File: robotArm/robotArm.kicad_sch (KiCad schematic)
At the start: 17 parts, among them J1 Barrel_Jack, J2 ENDSTOP INPUTS, J3 STEPPER1, J4 STEPPER4, J5 STEPPER2, J6 STEPPER3, SW1 SW_DIP_x08, SW2 SW_SPDT, U2 TMC2209_SILENTSTEPSTICK, U4 TMC2209_MODULE, U5 TMC2209 Module

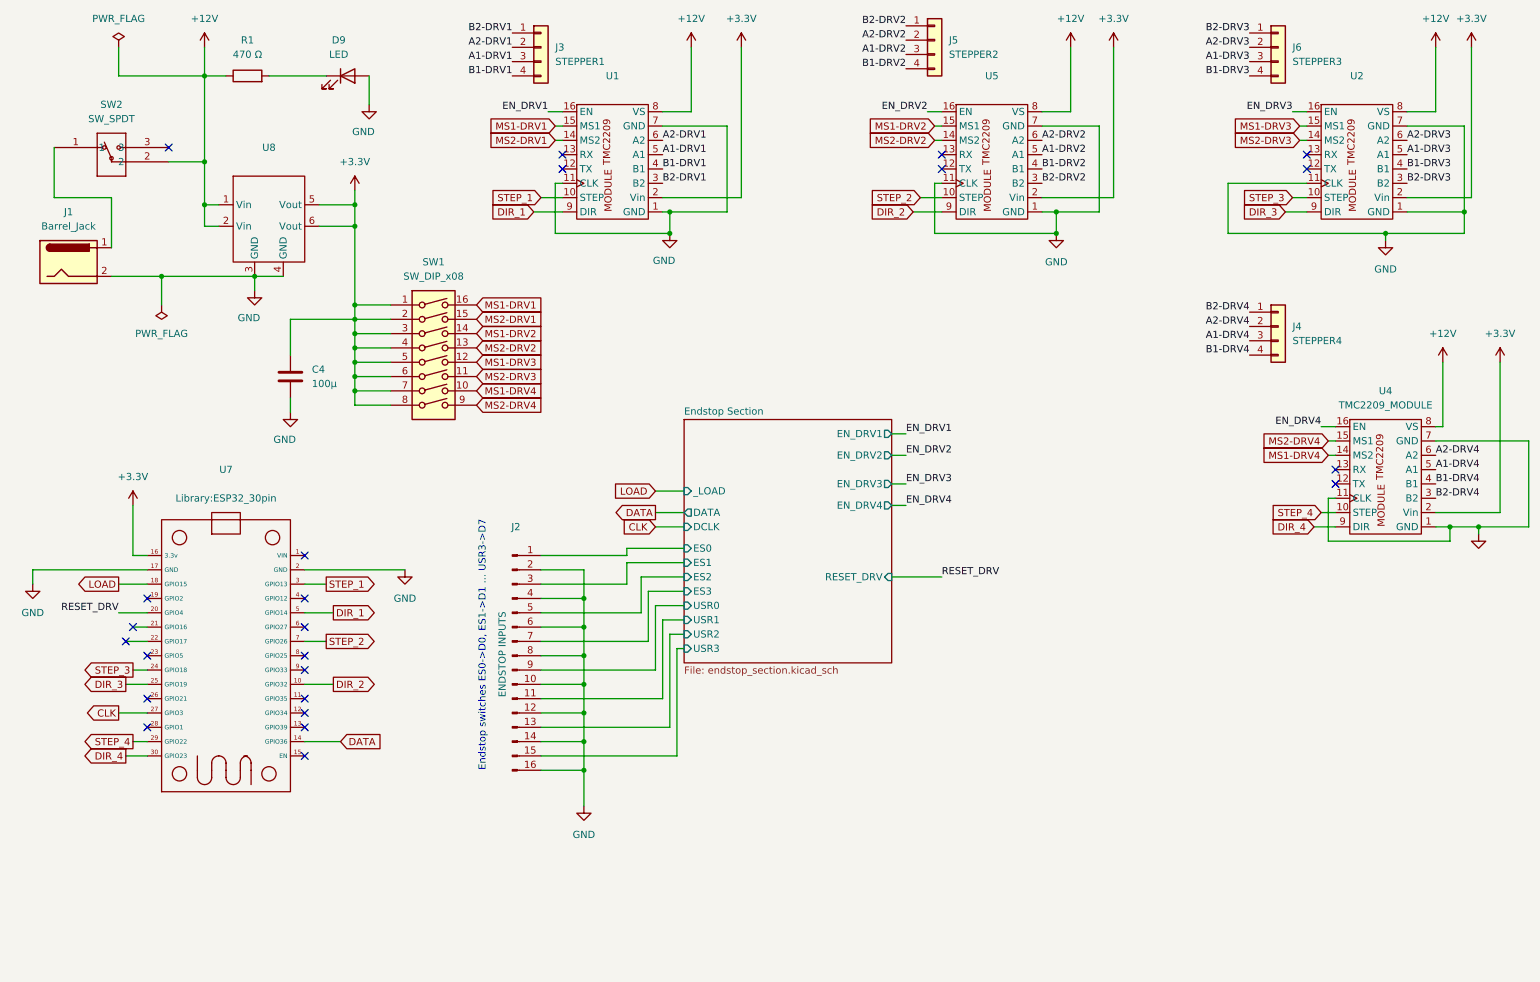
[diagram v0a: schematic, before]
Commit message: JLCPCB READY
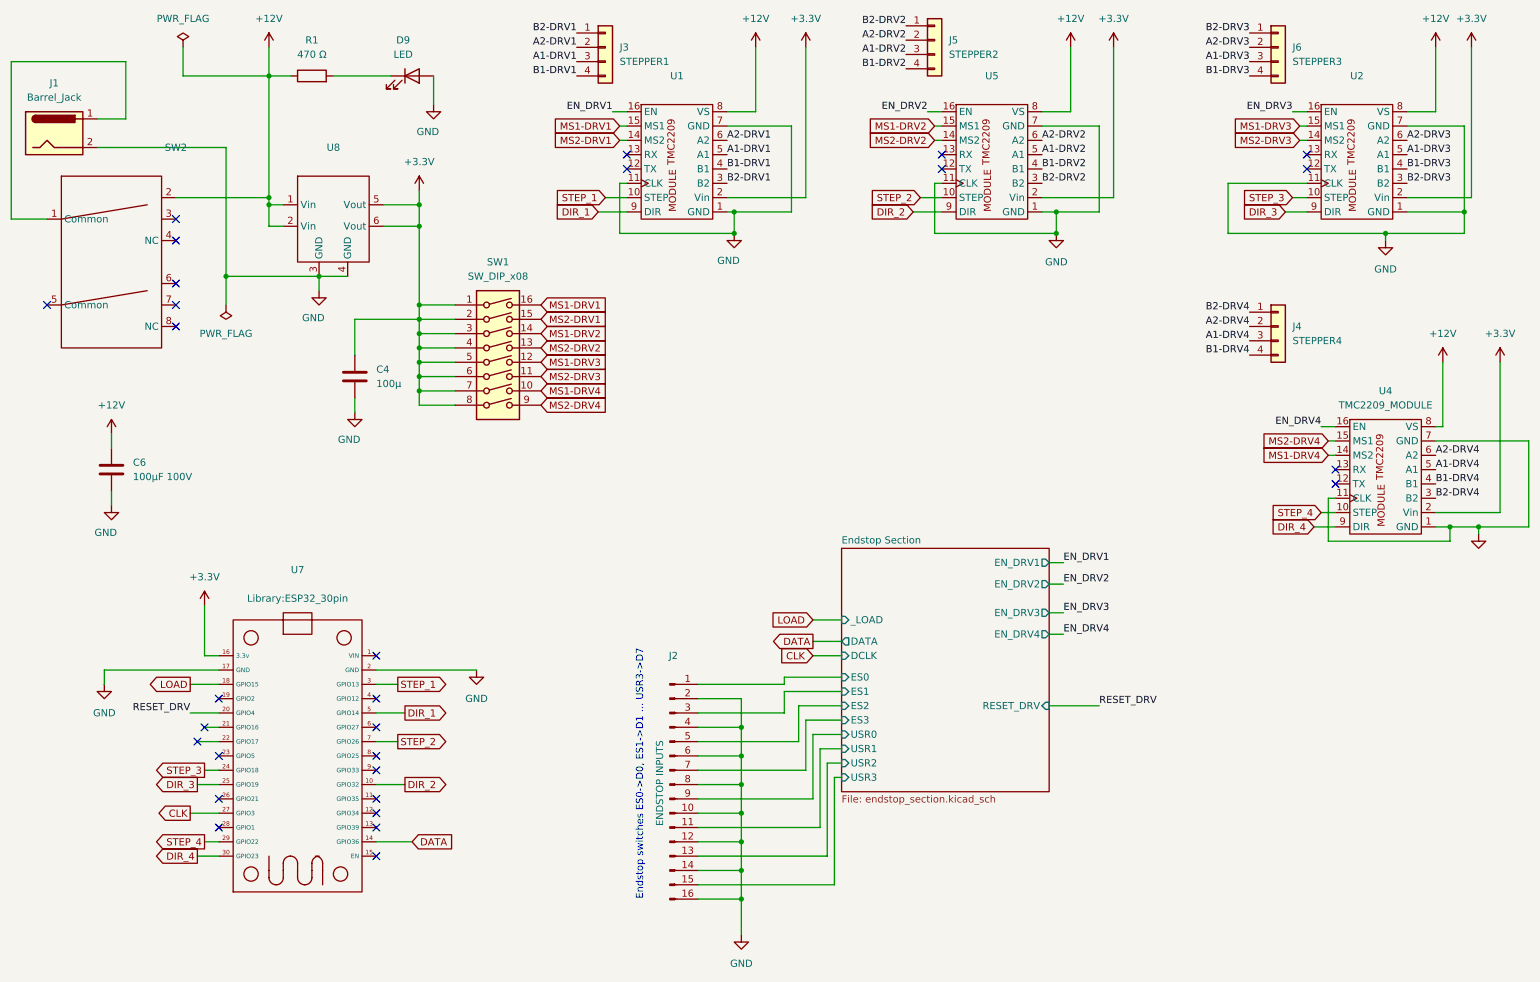
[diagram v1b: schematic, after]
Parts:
- removed SW2: SW_SPDT, SS-12D10G5_XKB, symbol 2026-09-22_07-48-55:SS-12D10G5
- added C6: 100µF 100V, Capacitor_THT:CP_Radial_D12.5mm_P2.50mm, symbol Device:C
- added SW2: ~, symbol K23D05_G6:2P3T
- SW1: footprint Package_DIP:DIP-16_W7.62mm -> Button_Switch_THT:SW_DIP_SPSTx08_Slide_6.7x21.88mm_W7.62mm_P2.54mm_LowProfile
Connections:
- net +12V: now also C6.1, SW2.2
- net GND: now also C6.2
- net at J1.1: now also SW2.1 (Common)
- no-connect marks 24 -> 29
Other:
- moved on the sheet: C4, D9, J1, J2, J3, R1, SW1, U1, U7, U8
